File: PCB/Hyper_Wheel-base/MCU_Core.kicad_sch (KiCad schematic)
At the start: 29 parts, among them U2 NRF52840-QIAA-R7, Y1 32MHz, Y2 Crystal

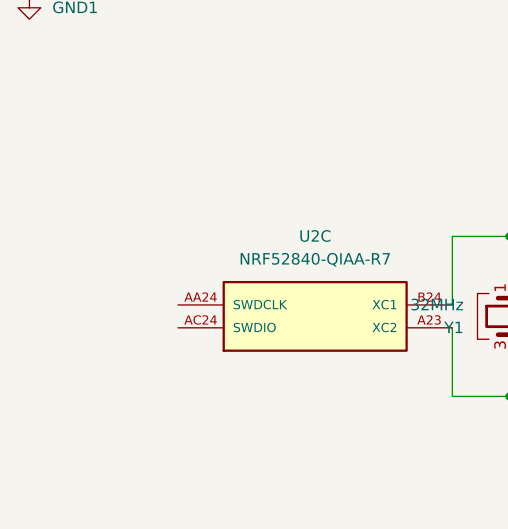
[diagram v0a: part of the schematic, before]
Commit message: Added test pads,
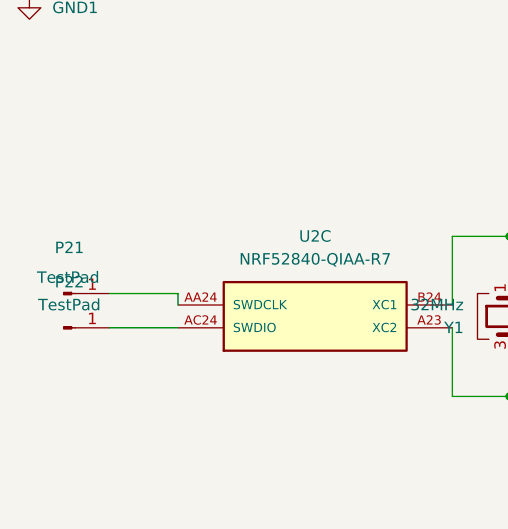
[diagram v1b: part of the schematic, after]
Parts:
- added P21, P22: TestPad, TestPoint:TestPoint_Pad_D2.0mm, symbol Connector:Conn_01x01_Pin
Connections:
- net at U2.AA24 (SWDCLK): now also P21.1 (Pin_1)
- net at U2.AC24 (SWDIO): now also P22.1 (Pin_1)
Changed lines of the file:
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@@
 	(wire
 		(pts
+			(xy 85.09 163.83) (xy 92.71 163.83)
+		)
+		(stroke
+			(width 0)
+			(type default)
+		)
+	)
+	(wire
+		(pts
 			(xy 138.43 157.48) (xy 138.43 166.37)
 		)
@@
 	(wire
 		(pts
+			(xy 85.09 167.64) (xy 92.71 167.64)
+		)
+		(stroke
+			(width 0)
+			(type default)
+		)
+	)
+	(wire
+		(pts
 			(xy 200.66 125.73) (xy 200.66 124.46)
 		)
@@
 	(wire
 		(pts
+			(xy 92.71 163.83) (xy 92.71 165.1)
+		)
+		(stroke
+			(width 0)
+			(type default)
+		)
+	)
+	(wire
+		(pts
 			(xy 76.2 124.46) (xy 76.2 130.81)
 		)
@@
 	)
 	(symbol
+		(lib_id "Connector:Conn_01x01_Pin")
+		(at 80.01 163.83 0)
+		(unit 1)
+		(body_style 1)
+		(exclude_from_sim no)
+		(in_bom yes)
+		(on_board yes)
+		(in_pos_files yes)
+		(dnp no)
+		(property "Reference" "P21"
+			(at 80.645 158.75 0)
+			(show_name no)
+			(do_not_autoplace no)
+			(effects
+				(font
+					(size 1.27 1.27)
+				)
+			)
+		)
+		(property "Value" "TestPad"
+			(at 80.518 162.052 0)
+			(show_name no)
+			(do_not_autoplace no)
+			(effects
+				(font
+					(size 1.27 1.27)
+				)
+			)
+		)
+		(property "Footprint" "TestPoint:TestPoint_Pad_D2.0mm"
+			(at 80.01 163.83 0)
+			(hide yes)
+			(show_name no)
+			(do_not_autoplace no)
+			(effects
+				(font
+					(size 1.27 1.27)
+				)
+			)
+		)
+		(property "Datasheet" ""
+			(at 80.01 163.83 0)
+			(hide yes)
+			(show_name no)
+			(do_not_autoplace no)
+			(effects
+				(font
+					(size 1.27 1.27)
+				)
+			)
+		)
+		(property "Description" "Generic connector, single row, 01x01, script generated"
+			(at 80.01 163.83 0)
+			(hide yes)
+			(show_name no)
+			(do_not_autoplace no)
+			(effects
+				(font
+					(size 1.27 1.27)
+				)
+			)
+		)
+		(pin "1"
+		)
+		(instances
+			(project "Hyper_Wheel-base"
+				(path "/3f05eeb1-03f9-49d1-8a58-0bc3d5427d25/11aa2f34-f9da-4218-833a-079f7b36f864"
+					(reference "P21")
+					(unit 1)
+				)
+			)
+		)
+	)
+	(symbol
 		(lib_id "power:GND")
 		(at 76.2 130.81 0)
@@
 					(unit 1)
 				)
+			)
+		)
+	)
+	(symbol
+		(lib_id "Connector:Conn_01x01_Pin")
+		(at 80.01 167.64 0)
+		(unit 1)
+		(body_style 1)
+		(exclude_from_sim no)
+		(in_bom yes)
+		(on_board yes)
+		(in_pos_files yes)
+		(dnp no)
+		(fields_autoplaced yes)
+		(property "Reference" "P22"
+			(at 80.645 162.56 0)
+			(show_name no)
+			(do_not_autoplace no)
+			(effects
+				(font
+					(size 1.27 1.27)
+				)
+			)
+		)
+		(property "Value" "TestPad"
+			(at 80.645 165.1 0)
+			(show_name no)
+			(do_not_autoplace no)
+			(effects
+				(font
+					(size 1.27 1.27)
+				)
+			)
+		)
+		(property "Footprint" "TestPoint:TestPoint_Pad_D2.0mm"
+			(at 80.01 167.64 0)
+			(hide yes)
+			(show_name no)
+			(do_not_autoplace no)
+			(effects
+				(font
+					(size 1.27 1.27)
+				)
+			)
+		)
+		(property "Datasheet" ""
+			(at 80.01 167.64 0)
+			(hide yes)
+			(show_name no)
+			(do_not_autoplace no)
+			(effects
+				(font
+					(size 1.27 1.27)
+				)
+			)
+		)
+		(property "Description" "Generic connector, single row, 01x01, script generated"
+			(at 80.01 167.64 0)
+			(hide yes)
+			(show_name no)
+			(do_not_autoplace no)
+			(effects
+				(font
+					(size 1.27 1.27)
+				)
+			)
+		)
+		(pin "1"
+		)
+		(instances
+			(project "Hyper_Wheel-base"
+				(path "/3f05eeb1-03f9-49d1-8a58-0bc3d5427d25/11aa2f34-f9da-4218-833a-079f7b36f864"
+					(reference "P22")
+					(unit 1)
+				)

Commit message: XIAO based test board complete
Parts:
- C1, C10, C11, C12, C13, C14, C15, C16, C17, C18, C19, C2, C20, C21, C22, C3, C4, C5, C6, C7, C8, C9, L1, L2, L3, L4: KiLib_Generator (none) -> SMD_2terminal_chip_molded
- P21, P22: footprint TestPoint:TestPoint_Pad_D2.0mm -> TestPoint:TestPoint_Pad_D1.0mm; now left out of the parts list
- Y1: KiLib_Generator (none) -> crystal_resonator_oscillator
